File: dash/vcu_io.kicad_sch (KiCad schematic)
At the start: 35 parts, among them J10 Conn_02x01, J11 Conn_02x02_Top_Bottom, J5 M80-5102042, J6 Conn_02x02_Top_Bottom, J7 Conn_02x01, J8 Conn_02x02_Top_Bottom, J9 Conn_02x01, Q2 XP262N7002TR-G, Q3 XP262N7002TR-G, Q4 XP262N7002TR-G, Q5 XP262N7002TR-G, U10 TCAN3404-Q1, U9 TCAN3404-Q1

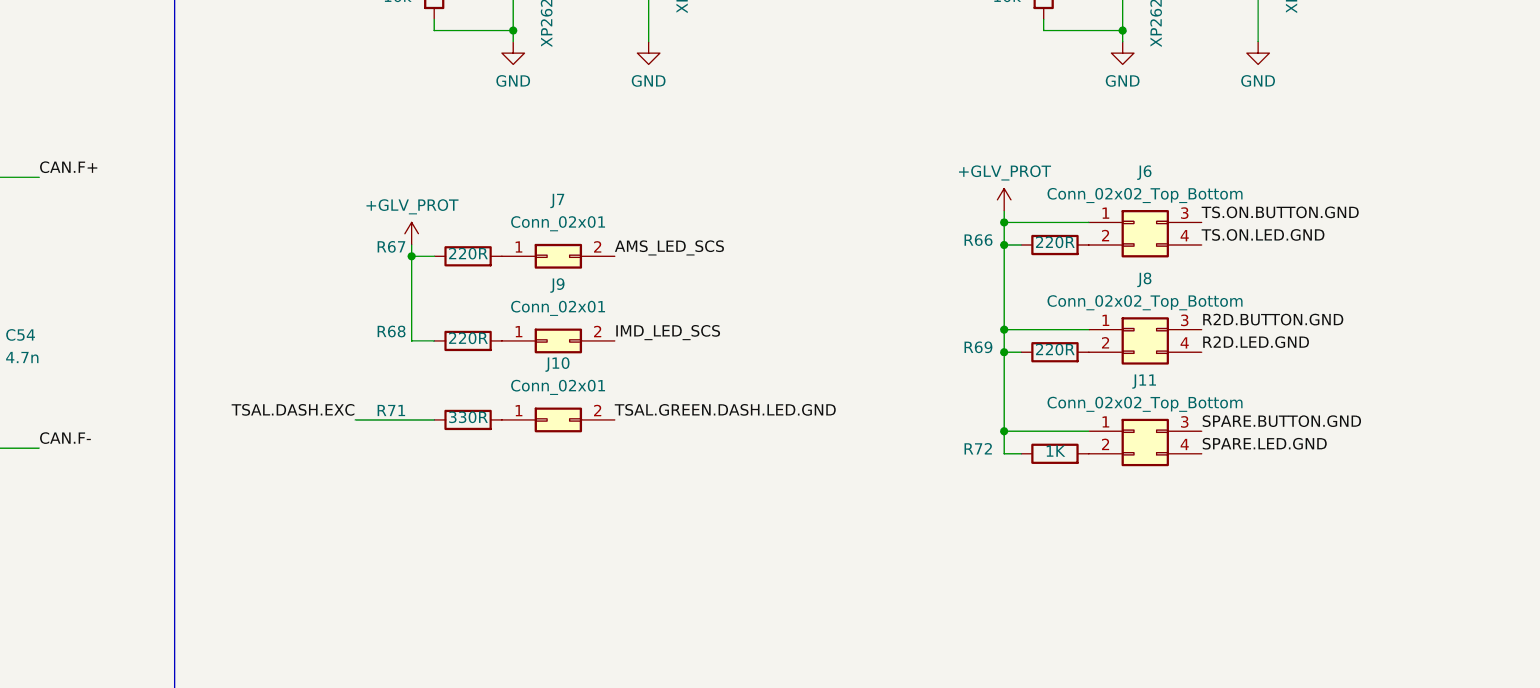
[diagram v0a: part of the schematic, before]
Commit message: finishing
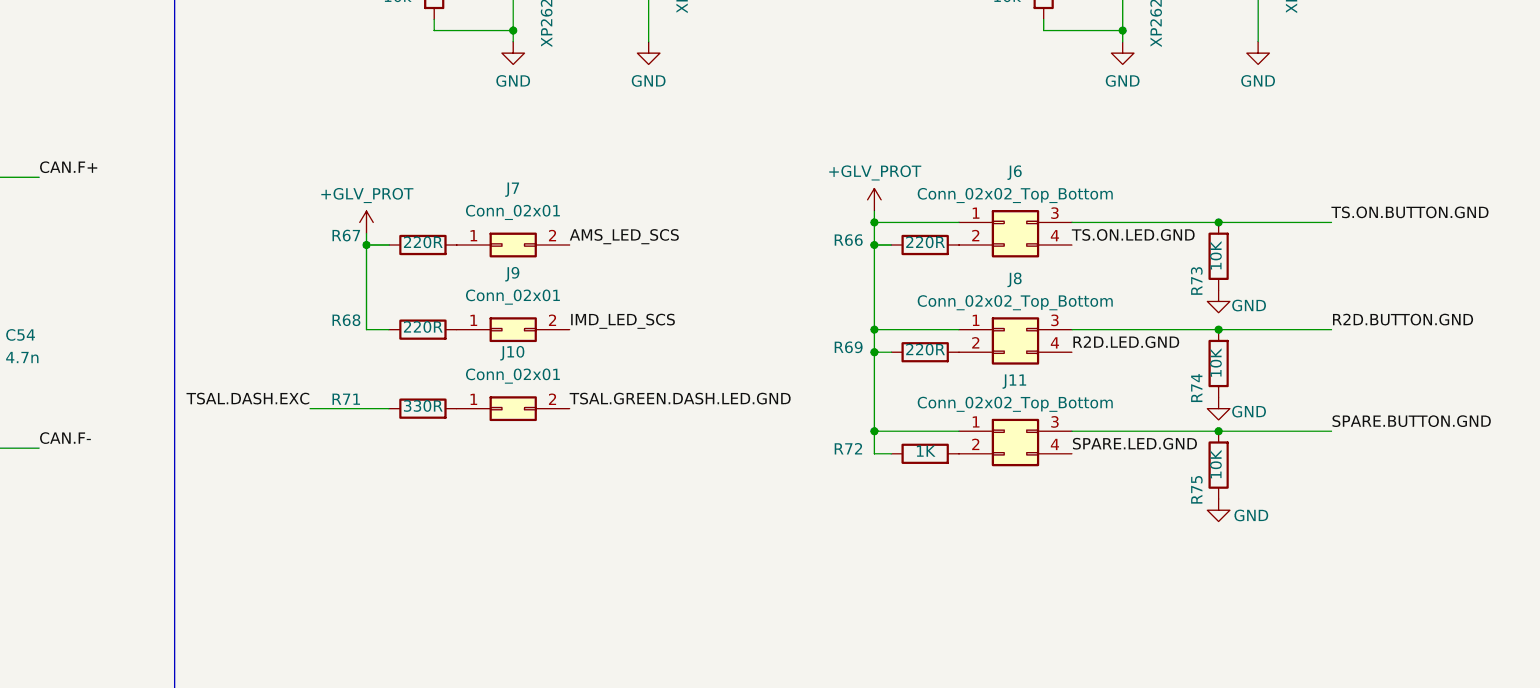
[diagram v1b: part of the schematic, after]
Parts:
- added R73, R74, R75: 10K, Resistor_SMD:R_0603_1608Metric, symbol Device:R
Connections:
- net GND: now also R73.1, R74.1, R75.1
- net R2D.BUTTON.GND: now also R74.2
- net SPARE.BUTTON.GND: now also R75.2
- net TS.ON.BUTTON.GND: now also R73.2
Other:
- moved on the sheet: J10, J11, J6, J7, J8, J9, R66, R67, R68, R69, R71, R72
